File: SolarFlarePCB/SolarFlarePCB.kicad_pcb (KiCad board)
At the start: 2 copper layers, 117.6 x 91.8 mm, 40 parts, among them U1 MOUDLE-SEEEDUINO-XIAO, U2 TRRS, U3 TRRS, U4 MOUDLE-SEEEDUINO-XIAO

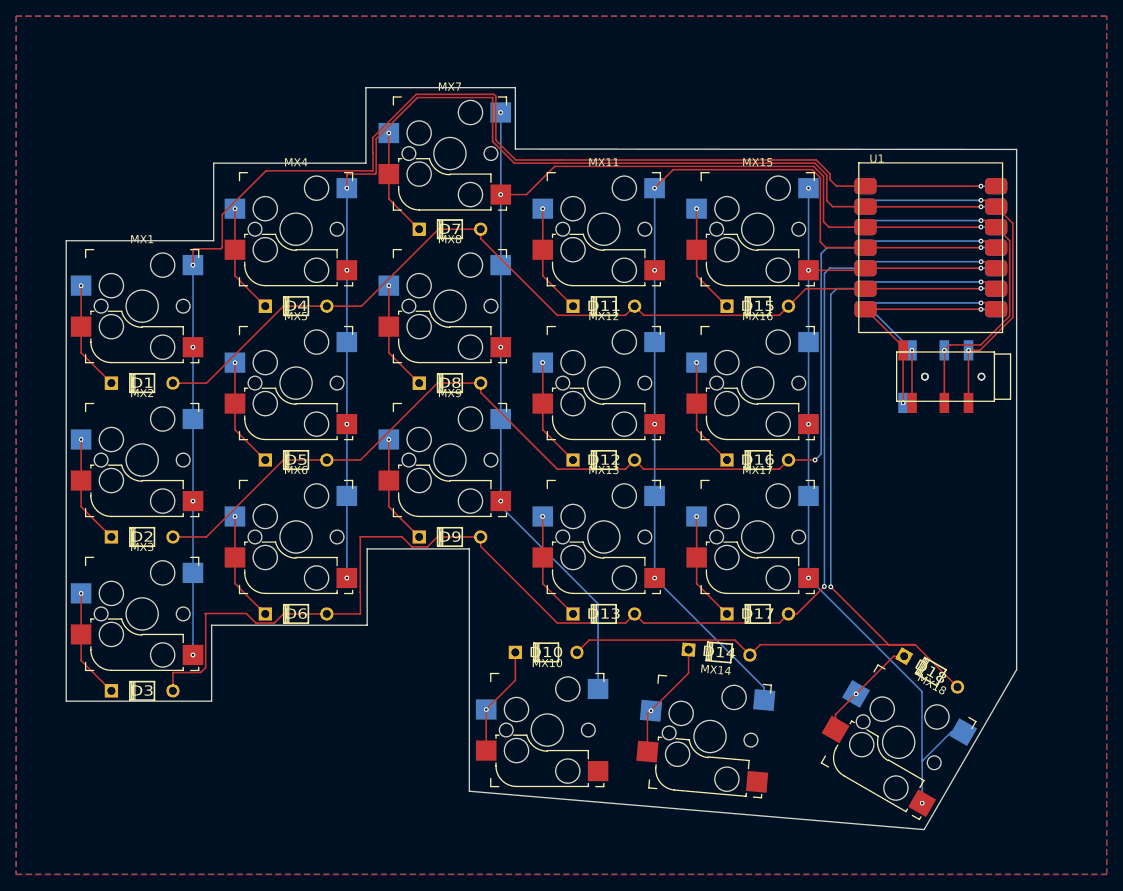
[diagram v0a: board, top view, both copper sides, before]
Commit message: starting to model
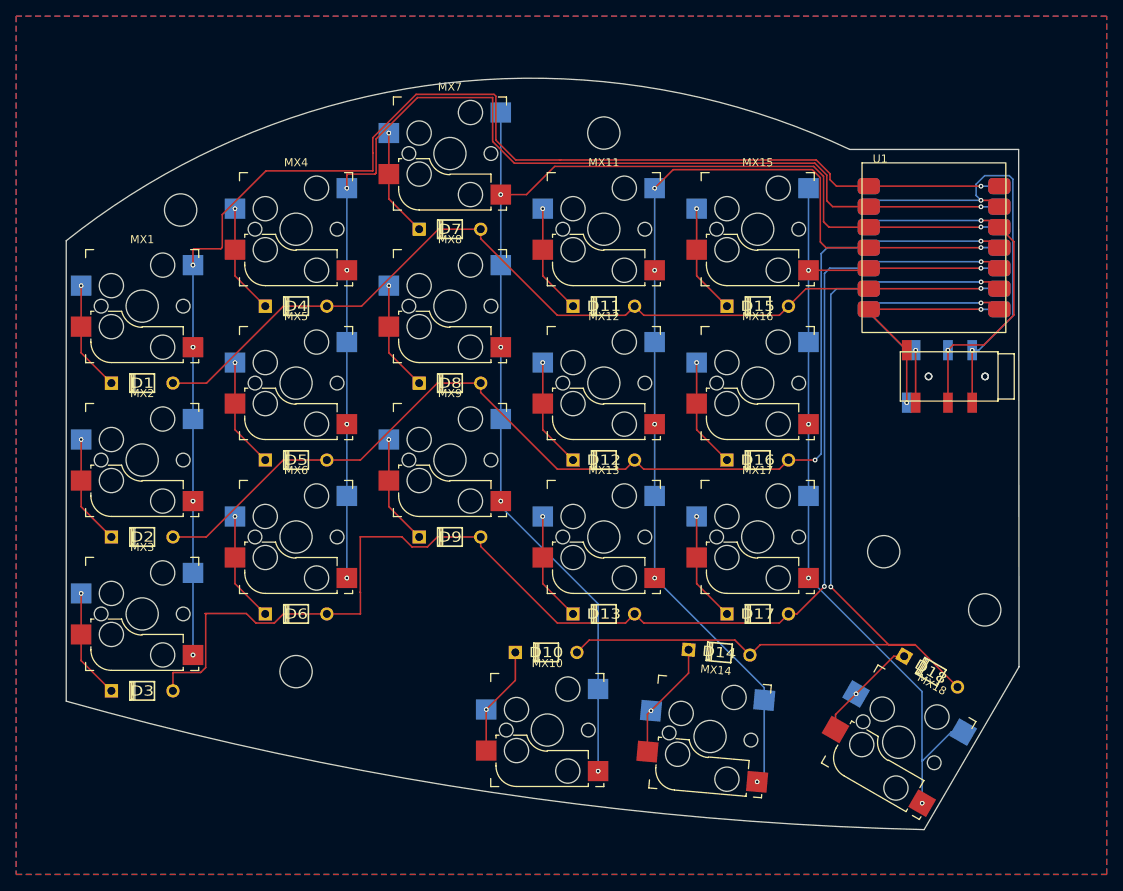
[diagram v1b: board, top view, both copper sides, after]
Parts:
- moved U2 0.45 mm to (144.1, 65.8)
- moved U3 0.45 mm to (144.1, 65.8)
- moved U1 0.40 mm to (127.2, 60.4)
- moved U4 0.40 mm to (145.1, 60.4)
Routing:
- net /col1: track 120.9 -> 131.4 mm, vias 5 -> 6
- net /col2: track 145.5 -> 155.7 mm
- net GND: track 45.1 -> 54.5 mm
- net /rx: track 31.2 -> 32.3 mm
- net /tx: track 29.7 -> 30.3 mm
- net /col0: vias 6 -> 5
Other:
- board size 117.6 x 91.8 mm -> 118 x 93 mm
